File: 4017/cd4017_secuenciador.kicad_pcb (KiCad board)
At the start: 2 copper layers, 71 x 47.5 mm, 19 parts, among them J1 Screw_Terminal_01x03, J2 Screw_Terminal_01x03, U1 CD4017BE

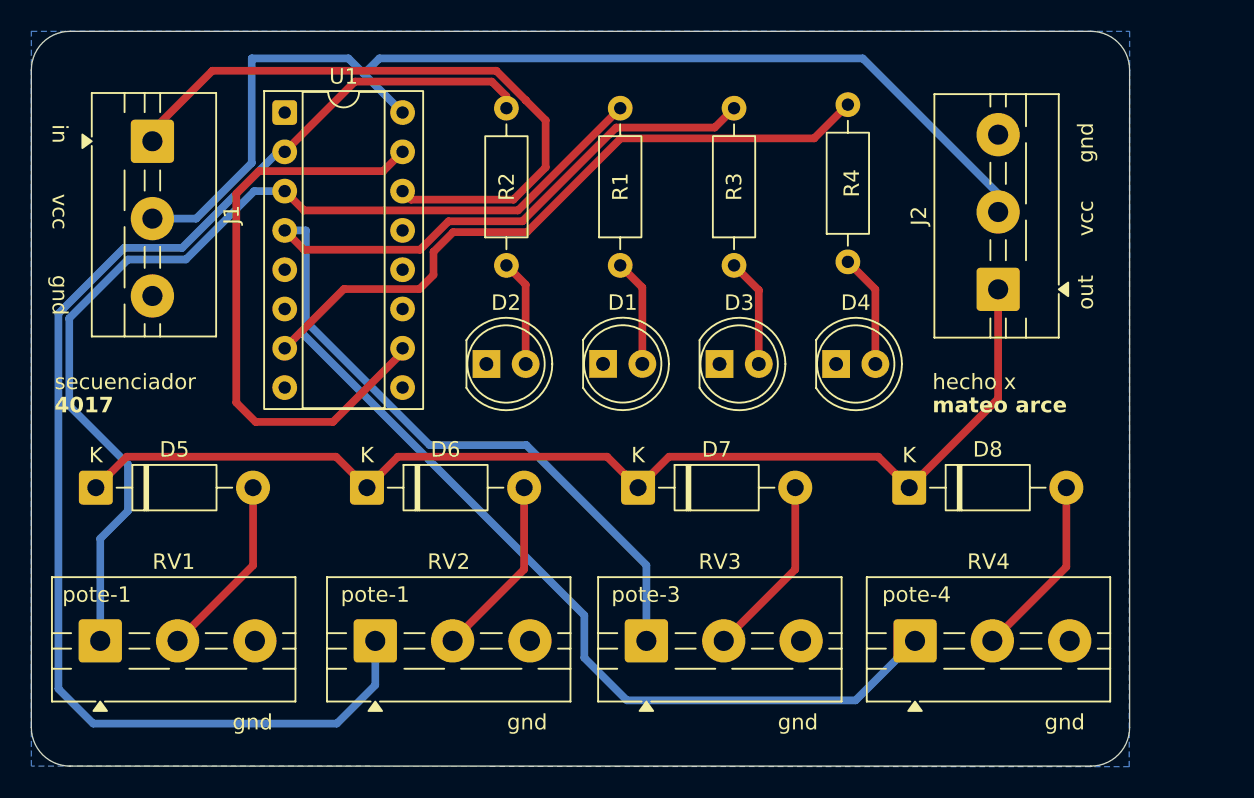
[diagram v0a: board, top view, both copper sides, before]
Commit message: gerbers + correcciones
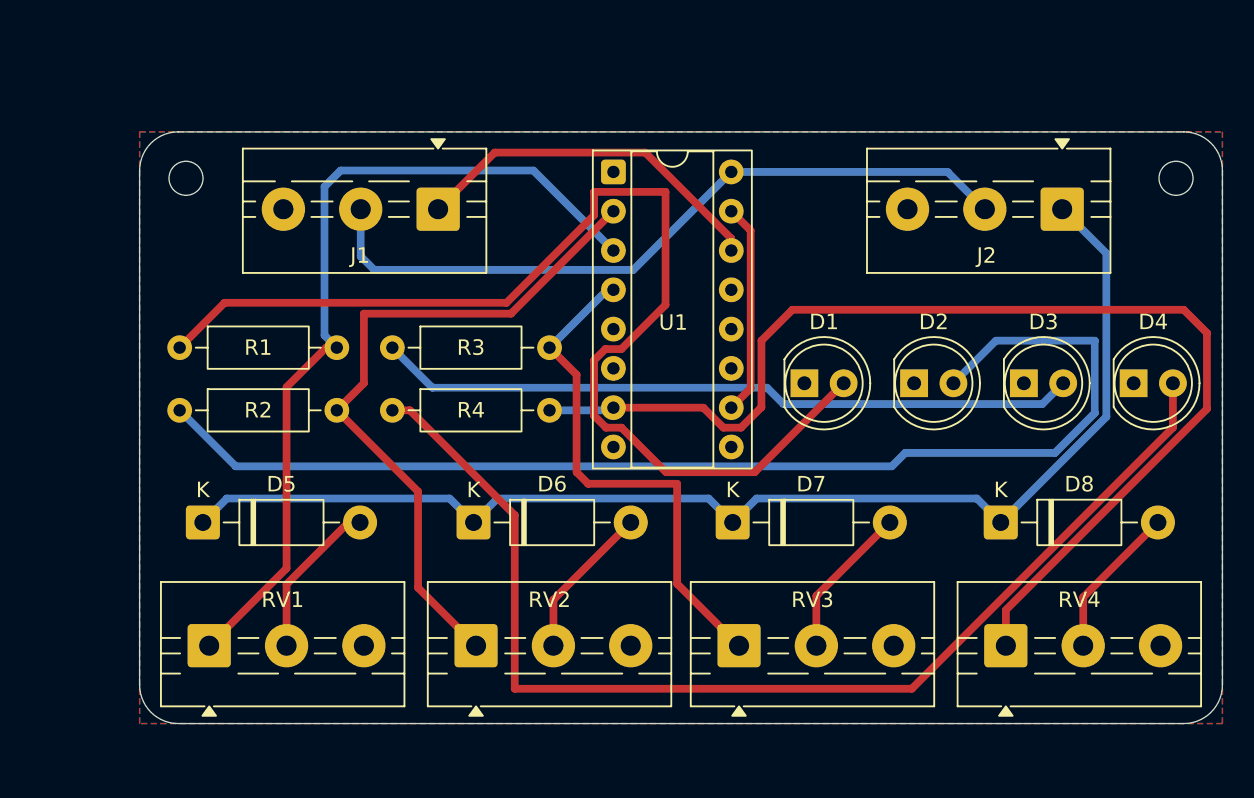
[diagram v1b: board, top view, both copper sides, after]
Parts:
- added REF**: MountingHole_2.2mm_M2, MountingHole:MountingHole_2.2mm_M2, F.Cu at (150.0, 99.5)
- added REF**: MountingHole_2.2mm_M2, MountingHole:MountingHole_2.2mm_M2, F.Cu at (214.0, 99.5)
- moved R4 31.0 mm to (163.3, 114.5), turned to 0 degrees
- moved R1 29.0 mm to (149.6, 110.5), turned to 0 degrees
- moved D2 27.7 mm to (197.1, 112.8)
- moved R2 23.1 mm to (149.6, 114.5), turned to 0 degrees
- moved R3 22.7 mm to (163.3, 110.5), turned to 0 degrees
- moved U1 21.6 mm to (177.6, 99.1)
- moved D3 19.7 mm to (204.2, 112.8)
- moved D4 19.3 mm to (211.3, 112.8)
- moved J1 19.0 mm to (166.3, 101.5), turned to 180 degrees
- moved D1 13.1 mm to (190.0, 112.8)
- moved D5 7.27 mm to (151.1, 121.8)
- moved D6 7.25 mm to (168.6, 121.8)
- moved RV1 7.05 mm to (151.5, 129.7)
- moved J2 6.63 mm to (206.6, 101.5), turned to 180 degrees
- moved RV2 6.52 mm to (168.8, 129.7)
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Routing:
- net Net-(D2-A): track 6.89 -> 77.0 mm
- net Net-(D4-A): track 7.34 -> 74.4 mm
- net Net-(D1-A): track 6.96 -> 73.5 mm
- net /Q1: track 85.9 -> 44.8 mm
- net /Q2: track 74.0 -> 33.4 mm
- net Net-(D3-A): track 7.04 -> 45.4 mm
- net Net-(U1-Q4): track 38.8 -> 13.7 mm
- net VCC: track 72.1 -> 47.4 mm
- net /Q3: track 98.1 -> 75.0 mm
- net Net-(J1-Pin_1): track 42.4 -> 23.5 mm
- net /Q0: track 65.5 -> 55.1 mm
- net Net-(D5-K): track 72.8 -> 79.7 mm
- net Net-(D8-A): track 11.9 -> 9.97 mm
- net Net-(D7-A): track 11.8 -> 9.94 mm
- net Net-(D6-A): track 11.8 -> 10.0 mm
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- added copper zone on F.Cu, net GND
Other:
- board size 71 x 47.5 mm -> 70 x 38.2 mm
- board text added: "secuenciador 4017"
- board text removed: "4017"
- board text removed: "gnd"
- board text removed: "hecho x"
- board text removed: "in"
- board text removed: "mateo arce"
- board text removed: "out"
- board text removed: "pote-1"
- board text removed: "pote-3"
- board text removed: "pote-4"
- board text removed: "secuenciador"
- board text removed: "vcc"
